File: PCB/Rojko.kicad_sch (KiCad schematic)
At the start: 35 parts, among them IC1 STM32L051C8T6, IC2 BQ25186DLHR, IC3 AP63203WU-7, J1 AYF-531035, J2 +, J3 -, J4 +, J5 -, J6 AYF-531035, SW1 SW_MEC_5G, U1 RYB080I, Y1 32,768k

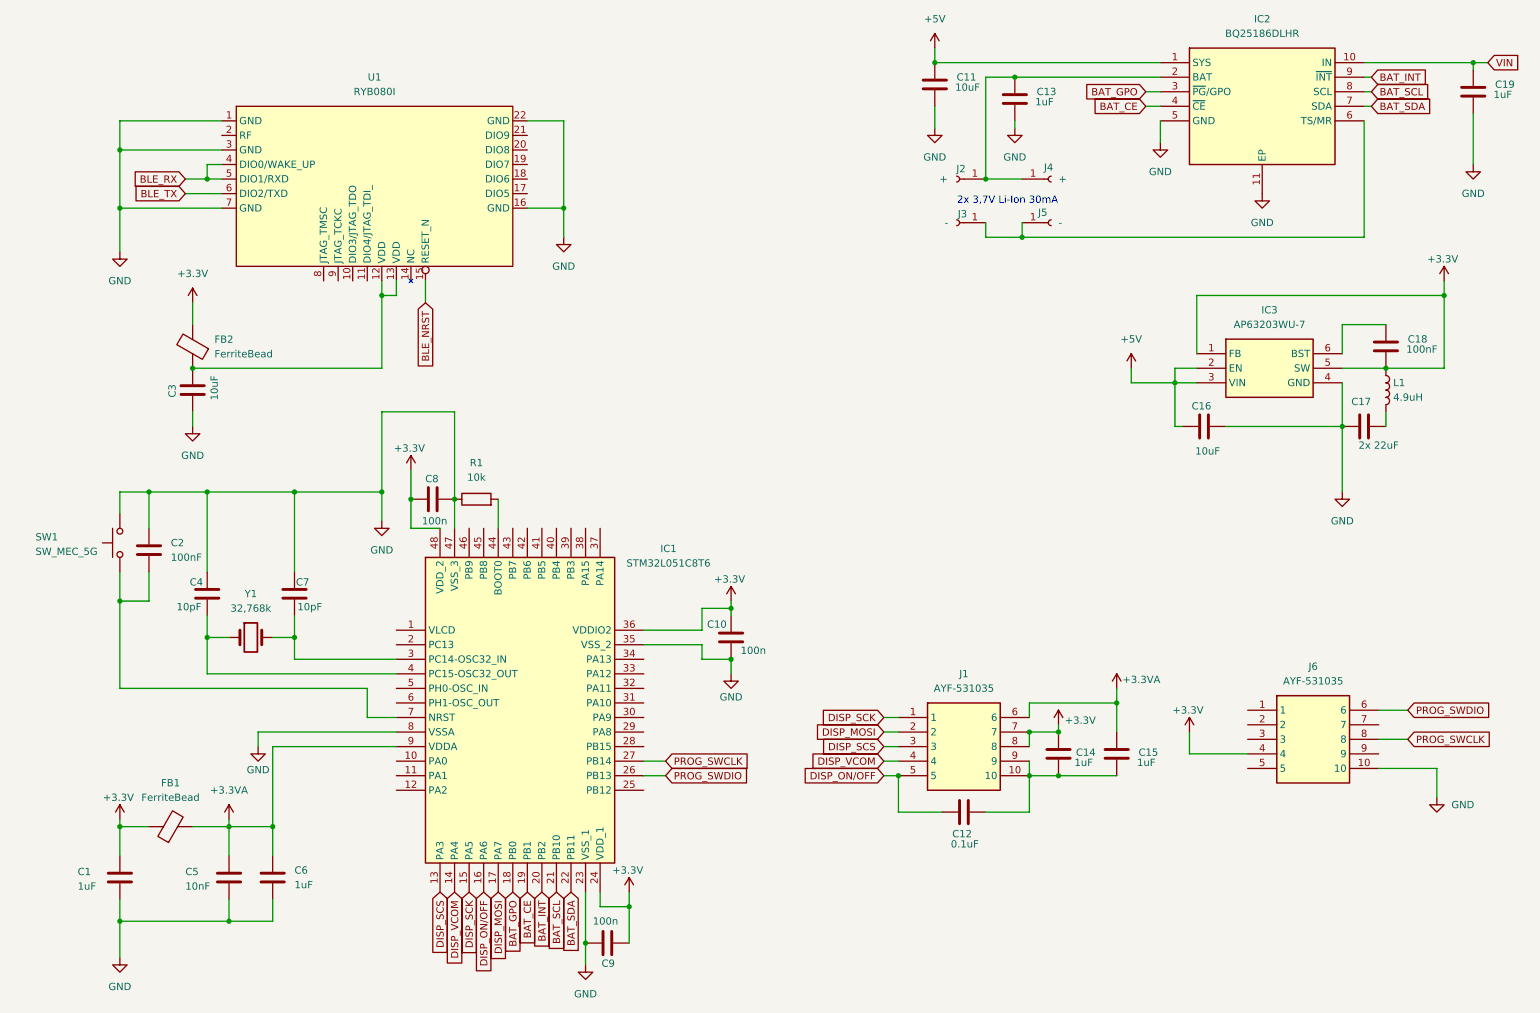
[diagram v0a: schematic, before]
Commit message: zmena chipu
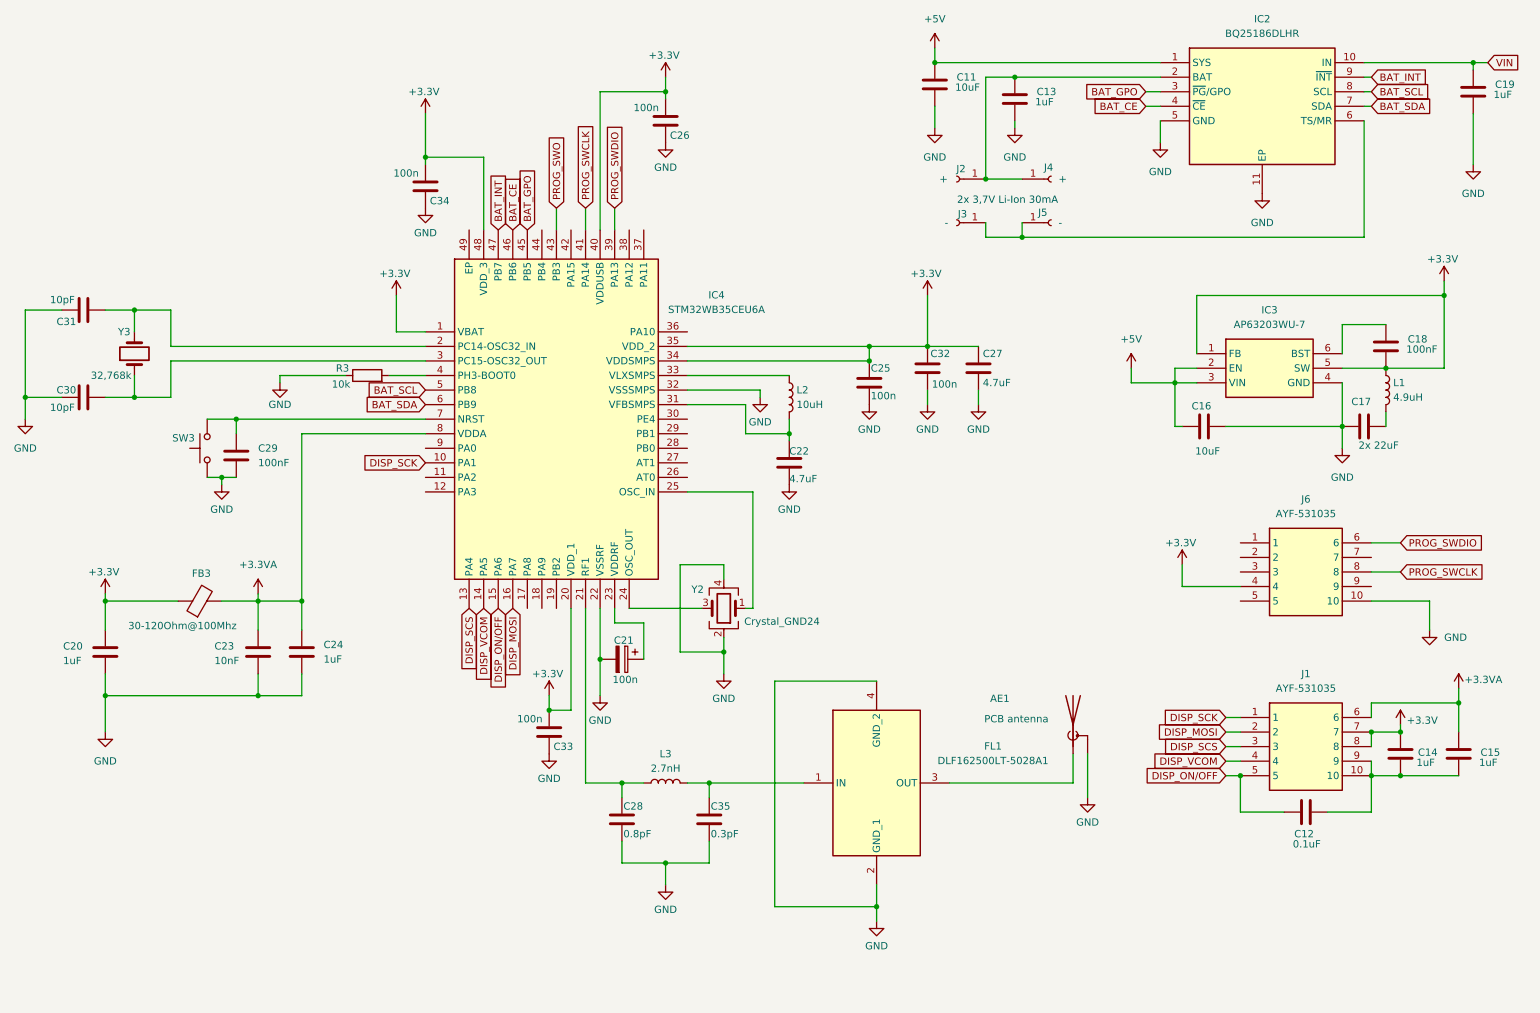
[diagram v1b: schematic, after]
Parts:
- removed C1, C6: 1uF, Capacitor_SMD:C_0201_0603Metric, symbol Device:C
- removed C10, C8, C9: 100n, Capacitor_SMD:C_0201_0603Metric, symbol Device:C
- removed C2: 100nF, Capacitor_SMD:C_0201_0603Metric, symbol Device:C
- removed C3: 10uF, Capacitor_SMD:C_0201_0603Metric, symbol Device:C
- removed C4, C7: 10pF, Capacitor_SMD:C_0201_0603Metric, symbol Device:C
- removed C5: 10nF, Capacitor_SMD:C_0201_0603Metric, symbol Device:C
- removed FB1: FerriteBead, Resistor_SMD:R_0805_2012Metric, symbol Device:FerriteBead
- removed FB2: FerriteBead, Resistor_SMD:R_0201_0603Metric, symbol Device:FerriteBead
- removed IC1: STM32L051C8T6, Package_QFP:LQFP-48_7x7mm_P0.5mm, symbol STM32L051C8T6:STM32L051C8T6
- removed R1: 10k, Resistor_SMD:R_0201_0603Metric, symbol Device:R
- removed SW1: SW_MEC_5G, CUSTOM:SWITCH small, symbol Switch:SW_MEC_5G
- removed U1: RYB080I, RYB080l:RYB080i, symbol RYB080l:RYB080i
- removed Y1: 32,768k, Crystal:Crystal_SMD_3215-2Pin_3.2x1.5mm, symbol Device:Crystal
- added AE1: PCB antenna, RF_Antenna:Texas_SWRA117D_2.4GHz_Right, symbol Device:Antenna_Shield
- added C20, C24: 1uF, Capacitor_SMD:C_0201_0603Metric, symbol Device:C
- added C21: 100n, symbol Device:C_Polarized
- added C22, C27: 4.7uF, Capacitor_SMD:C_0201_0603Metric, symbol Device:C
- added C23: 10nF, Capacitor_SMD:C_0201_0603Metric, symbol Device:C
- added C25, C26, C32, C33, C34: 100n, Capacitor_SMD:C_0201_0603Metric, symbol Device:C
- added C28: 0.8pF, symbol Device:C
- added C29: 100nF, Capacitor_SMD:C_0201_0603Metric, symbol Device:C
- added C30, C31: 10pF, Capacitor_SMD:C_0201_0603Metric, symbol Device:C
- added C35: 0.3pF, symbol Device:C
- added FB3: 30-120Ohm@100Mhz, Resistor_SMD:R_0805_2012Metric, symbol Device:FerriteBead
- added FL1: DLF162500LT-5028A1, DLF162500LT5028A1, symbol DLF162500LT-5028A1:DLF162500LT-5028A1
- added IC4: STM32WB35CEU6A, QFN50P700X700X60-49N-D, symbol STM32WB35CEU6A:STM32WB35CEU6A
- added L2: 10uH, symbol Device:L
- added L3: 2.7nH, symbol Device:L
- added R3: 10k, Resistor_SMD:R_0201_0603Metric, symbol Device:R
- added SW3: SW_MEC_5G, CUSTOM:SWITCH small, symbol Switch:SW_MEC_5G
- added Y2: Crystal_GND24, symbol Device:Crystal_GND24
- added Y3: 32,768k, Crystal:Crystal_SMD_3215-2Pin_3.2x1.5mm, symbol Device:Crystal
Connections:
- net +3.3V: now also C20.1, C25.1, C26.1, C27.1, C32.1, C33.1, C34.1, FB3.1, IC4.1 (VBAT), IC4.20 (VDD_1), IC4.34 (VDDSMPS), IC4.35 (VDD_2), IC4.40 (VDDUSB), IC4.48 (VDD_3)
- net +3.3VA: now also C23.1, C24.1, FB3.2, IC4.8 (VDDA)
- net BAT_CE: now also IC4.46 (PB6)
- net BAT_GPO: now also IC4.45 (PB5)
- net BAT_INT: now also IC4.47 (PB7)
- net BAT_SCL: now also IC4.5 (PB8)
- net BAT_SDA: now also IC4.6 (PB9)
- net DISP_MOSI: now also IC4.16 (PA7)
- net DISP_ON/OFF: now also IC4.15 (PA6)
- net DISP_SCK: now also IC4.10 (PA1)
- net DISP_SCS : now also IC4.13 (PA4)
- net DISP_VCOM: now also IC4.14 (PA5)
- net GND: now also AE1.2 (Shield), C20.2, C21.2, C22.2, C23.2, C24.2, C25.2, C26.2, C27.2, C28.2, C29.1, C30.1, C31.1, C32.2, C33.2, C34.2, C35.2, FL1.2 (GND_1), FL1.4 (GND_2), IC4.22 (VSSRF), IC4.32 (VSSSMPS), R3.1, SW3.1 (A), SW3.2 (A), Y2.2, Y2.4
- net PROG_SWCLK: now also IC4.41 (PA14)
- net PROG_SWDIO: now also IC4.39 (PA13)
- new net: C21.1, IC4.23 (VDDRF)
- new net: C35.1, FL1.1 (IN), L3.2
- new net: AE1.1 (A), FL1.3 (OUT)
- new net: C31.2, IC4.2 (PC14-OSC32_IN), Y3.2
- new net: C22.1, IC4.31 (VFBSMPS), L2.2
- new net: C30.2, IC4.3 (PC15-OSC32_OUT), Y3.1
- new net: C29.2, IC4.7 (NRST), SW3.3 (B), SW3.4 (B)
- new net: IC4.33 (VLXSMPS), L2.1
- new net: IC4.4 (PH3-BOOT0), R3.2
- new net: IC4.25 (OSC_IN), Y2.1
- new net: IC4.24 (OSC_OUT), Y2.3
- new net: C28.1, IC4.21 (RF1), L3.1
- new net PROG_SWO: IC4.43 (PB3)
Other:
- moved on the sheet: C12, C14, C15, J1, J6
